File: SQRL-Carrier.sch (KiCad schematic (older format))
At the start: 59 parts, among them J1 M.2_M-key, J2 PCIE-164-02-F-D-RA, J3 4-Pin Molex, U1 DSC1104, U2 SI53322, U3 TPS563231, U4 TPS563231, U5 spoolqueue_logo

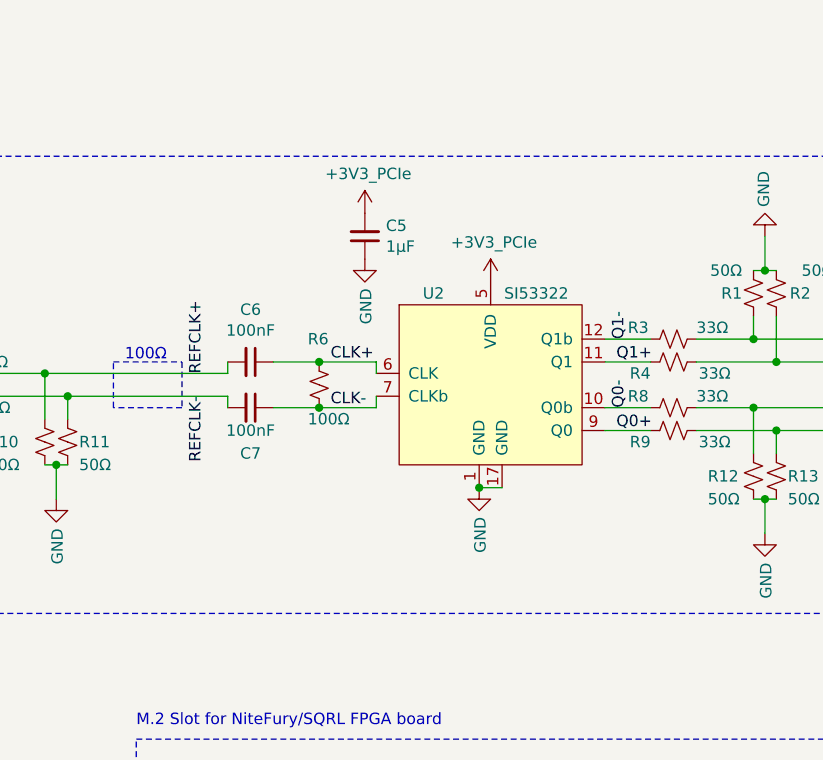
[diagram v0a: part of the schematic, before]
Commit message: Hardware revision 2
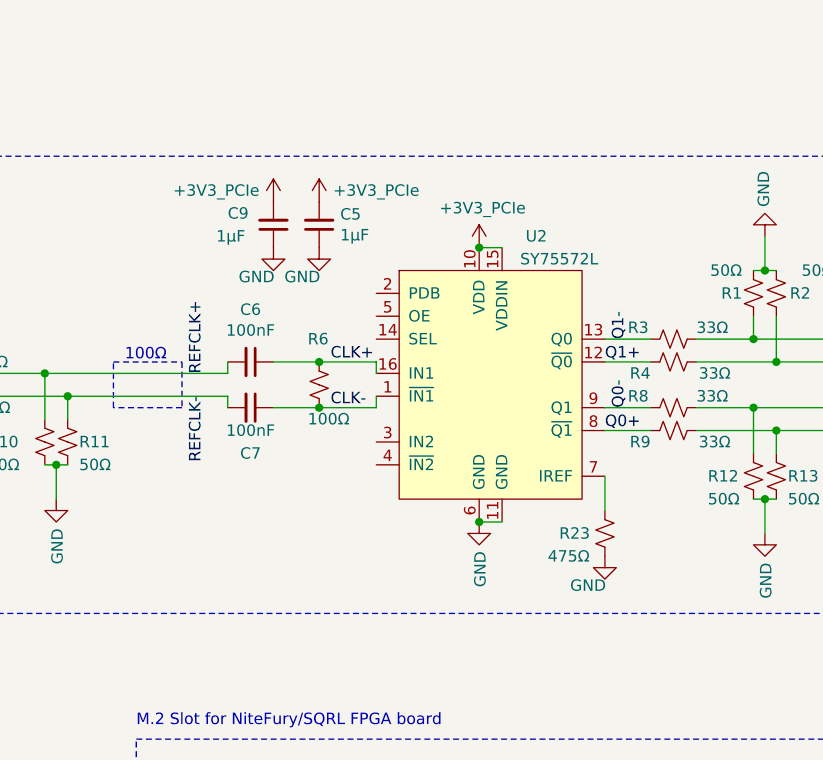
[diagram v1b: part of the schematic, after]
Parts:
- removed U2: SI53322, Package_DFN_QFN:VQFN-16-1EP_3x3mm_P0.5mm_EP1.68x1.68mm_ThermalVias, symbol PCIe_Clock:SI53322
- added C9: 1μF, Capacitor_SMD:C_0402_1005Metric, symbol Device:C_Small
- added R23: 475Ω, Resistor_SMD:R_0402_1005Metric, symbol Device:R_Small_US
- added U2: SY75572L, Package_DFN_QFN:VQFN-16-1EP_3x3mm_P0.5mm_EP1.45x1.45mm, symbol PCIe_Clock:SY75572L
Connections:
- net +3V3_PCIe: now also C9.2, U2.10 (VDD), U2.15 (VDDIN)
- net CLK+: now also U2.16 (IN1)
- net CLK-: now also U2.1 (~IN1~)
- net GND: now also C9.1, R23.2, U2.11 (GND), U2.6 (GND)
- net Q0+: now also U2.8 (~Q1~)
- net Q0-: now also U2.9 (Q1)
- net Q1+: now also U2.12 (~Q0~)
- net Q1-: now also U2.13 (Q0)
- new net: R23.1, U2.7 (IREF)
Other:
- moved on the sheet: C5
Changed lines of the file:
@@
 L power:GND #PWR0114
 U 1 1 5EADCD70
-P 8000 3450
-F 0 "#PWR0114" H 8000 3200 50  0001 C CNN
-F 1 "GND" V 8005 3322 50  0000 R CNN
-F 2 "" H 8000 3450 50  0001 C CNN
-F 3 "" H 8000 3450 50  0001 C CNN
-	1    8000 3450
+P 8000 3600
+F 0 "#PWR0114" H 8000 3350 50  0001 C CNN
+F 1 "GND" V 8005 3472 50  0000 R CNN
+F 2 "" H 8000 3600 50  0001 C CNN
+F 3 "" H 8000 3600 50  0001 C CNN
+	1    8000 3600
 	1    0    0    -1
 $EndComp
@@
 Wire Wire Line
 	11200 6000 11300 6000
-$Comp
-L PCIe_Clock:SI53322 U2
-U 1 1 5EB6B52B
-P 8050 3000
-F 0 "U2" H 7800 3400 50  0000 C CNN
-F 1 "SI53322" H 8250 3400 50  0000 C CNN
-F 2 "Package_DFN_QFN:VQFN-16-1EP_3x3mm_P0.5mm_EP1.68x1.68mm_ThermalVias" H 8050 3000 50  0001 C CNN
-F 3 "" H 8050 3000 50  0001 C CNN
-	1    8050 3000
-	1    0    0    -1
-$EndComp
-Wire Wire Line
-	8000 3450 8100 3450
-Connection ~ 8000 3450
+Wire Wire Line
+	8000 3600 8100 3600
 $Comp
 L power:GND #PWR0115
@@
 	6200 3050 6900 3050
 $Comp
-L Device:R_Small_US R12
-U 1 1 5EBAFF1E
-P 9200 3400
-F 0 "R12" H 9000 3400 50  0000 L CNN
-F 1 "50Ω" H 9000 3300 50  0000 L CNN
-F 2 "Resistor_SMD:R_0402_1005Metric" H 9200 3400 50  0001 C CNN
-F 3 "~" H 9200 3400 50  0001 C CNN
-	1    9200 3400
-	1    0    0    -1
-$EndComp
-$Comp
-L Device:R_Small_US R13
-U 1 1 5EBAFF24
-P 9300 3400
-F 0 "R13" H 9350 3400 50  0000 L CNN
-F 1 "50Ω" H 9350 3300 50  0000 L CNN
-F 2 "Resistor_SMD:R_0402_1005Metric" H 9300 3400 50  0001 C CNN
-F 3 "~" H 9300 3400 50  0001 C CNN
-	1    9300 3400
-	1    0    0    -1
-$EndComp
-$Comp
 L power:GND #PWR0117
 U 1 1 5EBAFF2A
@@
 	9200 3500 9250 3500
 Connection ~ 9250 3500
-$Comp
-L Device:R_Small_US R8
-U 1 1 5EBAFF34
-P 8850 3100
-F 0 "R8" V 8800 2900 50  0000 L CNN
-F 1 "33Ω" V 8800 3200 50  0000 L CNN
-F 2 "Resistor_SMD:R_0402_1005Metric" H 8850 3100 50  0001 C CNN
-F 3 "~" H 8850 3100 50  0001 C CNN
-	1    8850 3100
-	0    1    1    0
-$EndComp
-$Comp
-L Device:R_Small_US R9
-U 1 1 5EBAFF3A
-P 8850 3200
-F 0 "R9" V 8800 3300 50  0000 L CNN
-F 1 "33Ω" V 8800 2950 50  0000 L CNN
-F 2 "Resistor_SMD:R_0402_1005Metric" H 8850 3200 50  0001 C CNN
-F 3 "~" H 8850 3200 50  0001 C CNN
-	1    8850 3200
-	0    -1   -1   0
-$EndComp
 Wire Wire Line
 	8550 3100 8750 3100
@@
 Wire Wire Line
 	9300 3200 10050 3200
-$Comp
-L Device:R_Small_US R2
-U 1 1 5EBC0DFE
-P 9300 2600
-F 0 "R2" H 9150 2600 50  0000 L CNN
-F 1 "50Ω" H 9050 2500 50  0000 L CNN
-F 2 "Resistor_SMD:R_0402_1005Metric" H 9300 2600 50  0001 C CNN
-F 3 "~" H 9300 2600 50  0001 C CNN
-	1    9300 2600
-	-1   0    0    1
-$EndComp
-$Comp
-L Device:R_Small_US R1
-U 1 1 5EBC0E04
-P 9200 2600
-F 0 "R1" H 9250 2600 50  0000 L CNN
-F 1 "50Ω" H 9250 2500 50  0000 L CNN
-F 2 "Resistor_SMD:R_0402_1005Metric" H 9200 2600 50  0001 C CNN
-F 3 "~" H 9200 2600 50  0001 C CNN
-	1    9200 2600
-	-1   0    0    1
-$EndComp
 $Comp
 L power:GND #PWR0118
@@
 Wire Wire Line
 	9300 2900 10050 2900
-$Comp
-L Device:R_Small_US R4
-U 1 1 5EBC0E14
-P 8850 2900
-F 0 "R4" V 8800 3000 50  0000 L CNN
-F 1 "33Ω" V 8800 2650 50  0000 L CNN
-F 2 "Resistor_SMD:R_0402_1005Metric" H 8850 2900 50  0001 C CNN
-F 3 "~" H 8850 2900 50  0001 C CNN
-	1    8850 2900
-	0    -1   -1   0
-$EndComp
 Wire Wire Line
 	8750 2900 8550 2900
 Wire Wire Line
 	8550 2800 8750 2800
-$Comp
-L Device:R_Small_US R3
-U 1 1 5EBC0E1A
-P 8850 2800
-F 0 "R3" V 8800 2600 50  0000 L CNN
-F 1 "33Ω" V 8800 2900 50  0000 L CNN
-F 2 "Resistor_SMD:R_0402_1005Metric" H 8850 2800 50  0001 C CNN
-F 3 "~" H 8850 2800 50  0001 C CNN
-	1    8850 2800
-	0    1    1    0
-$EndComp
 Wire Notes Line
 	9550 3050 9850 3050
@@
 L Device:C_Small C5
 U 1 1 5EEDCC6E
-P 7500 2350
-F 0 "C5" H 7408 2304 50  0000 R CNN
-F 1 "1μF" H 7408 2395 50  0000 R CNN
-F 2 "Capacitor_SMD:C_0402_1005Metric" H 7500 2350 50  0001 C CNN
-F 3 "~" H 7500 2350 50  0001 C CNN
-	1    7500 2350
+P 7300 2300
+F 0 "C5" H 7208 2254 50  0000 R CNN
+F 1 "1μF" H 7208 2345 50  0000 R CNN
+F 2 "Capacitor_SMD:C_0402_1005Metric" H 7300 2300 50  0001 C CNN
+F 3 "~" H 7300 2300 50  0001 C CNN
+	1    7300 2300
 	-1   0    0    1
-$EndComp
-$Comp
-L power:GND #PWR0225
-U 1 1 5EEDCC74
-P 7500 2450
-F 0 "#PWR0225" H 7500 2200 50  0001 C CNN
-F 1 "GND" V 7505 2322 50  0000 R CNN
-F 2 "" H 7500 2450 50  0001 C CNN
-F 3 "" H 7500 2450 50  0001 C CNN
-	1    7500 2450
-	1    0    0    -1
 $EndComp
 $Comp
 L Carrier_power:+3V3_PCIe #PWR0226
 U 1 1 5EEE3C1E
-P 8050 2550
-F 0 "#PWR0226" H 8050 2400 50  0001 C CNN
-F 1 "+3V3_PCIe" H 8065 2723 50  0000 C CNN
-F 2 "" H 8050 2550 50  0001 C CNN
-F 3 "" H 8050 2550 50  0001 C CNN
-	1    8050 2550
+P 8000 2400
+F 0 "#PWR0226" H 8000 2250 50  0001 C CNN
+F 1 "+3V3_PCIe" H 8015 2573 50  0000 C CNN
+F 2 "" H 8000 2400 50  0001 C CNN
+F 3 "" H 8000 2400 50  0001 C CNN
+	1    8000 2400
 	1    0    0    -1
 $EndComp
@@
 L Carrier_power:+3V3_PCIe #PWR0227
 U 1 1 5EEE78B2
-P 7500 2250
-F 0 "#PWR0227" H 7500 2100 50  0001 C CNN
-F 1 "+3V3_PCIe" H 7515 2423 50  0000 C CNN
-F 2 "" H 7500 2250 50  0001 C CNN
-F 3 "" H 7500 2250 50  0001 C CNN
-	1    7500 2250
+P 7300 2200
+F 0 "#PWR0227" H 7300 2050 50  0001 C CNN
+F 1 "+3V3_PCIe" H 7550 2250 50  0000 C CNN
+F 2 "" H 7300 2200 50  0001 C CNN
+F 3 "" H 7300 2200 50  0001 C CNN
+	1    7300 2200
 	1    0    0    -1
 $EndComp
@@
 Text Label 8650 2800 1    50   ~ 0
 Q1-
-Text Label 8600 2900 0    50   ~ 0
+Text Label 8550 2900 0    50   ~ 0
 Q1+
-Text Label 8600 3200 0    50   ~ 0
+Text Label 8550 3200 0    50   ~ 0
 Q0+
 Text Label 8650 3100 1    50   ~ 0
@@
 	1    0    0    -1
 $EndComp
+$Comp
+L PCIe_Clock:SY75572L U2
+U 1 1 5F5400E1
+P 8050 3000
+F 0 "U2" H 8250 3650 50  0000 C CNN
+F 1 "SY75572L" H 8350 3550 50  0000 C CNN
+F 2 "Package_DFN_QFN:VQFN-16-1EP_3x3mm_P0.5mm_EP1.45x1.45mm" H 8050 3000 50  0001 C CNN
+F 3 "" H 8050 3000 50  0001 C CNN
+	1    8050 3000
+	1    0    0    -1
+$EndComp
+Connection ~ 8000 3600
+Wire Wire Line
+	8000 2400 8100 2400
+Connection ~ 8000 2400
+$Comp
+L Device:R_Small_US R23
+U 1 1 5F59552E
+P 8550 3650
+F 0 "R23" H 8350 3650 50  0000 L CNN
+F 1 "475Ω" H 8300 3550 50  0000 L CNN
+F 2 "Resistor_SMD:R_0402_1005Metric" H 8550 3650 50  0001 C CNN
+F 3 "~" H 8550 3650 50  0001 C CNN
+	1    8550 3650
+	1    0    0    -1
+$EndComp
+$Comp
+L power:GND #PWR0240
+U 1 1 5F597145
+P 8550 3750
+F 0 "#PWR0240" H 8550 3500 50  0001 C CNN
+F 1 "GND" H 8555 3622 50  0000 R CNN
+F 2 "" H 8550 3750 50  0001 C CNN
+F 3 "" H 8550 3750 50  0001 C CNN
+	1    8550 3750
+	1    0    0    -1
+$EndComp
+Wire Wire Line
+	8550 3550 8550 3400
+$Comp
+L Device:R_Small_US R8
+U 1 1 5EBAFF34
+P 8850 3100
+F 0 "R8" V 8800 2900 50  0000 L CNN
+F 1 "33Ω" V 8800 3200 50  0000 L CNN
+F 2 "Resistor_SMD:R_0402_1005Metric" H 8850 3100 50  0001 C CNN
+F 3 "~" H 8850 3100 50  0001 C CNN
+	1    8850 3100
+	0    1    1    0
+$EndComp
+$Comp
+L Device:R_Small_US R9
+U 1 1 5EBAFF3A
+P 8850 3200
+F 0 "R9" V 8800 3300 50  0000 L CNN
+F 1 "33Ω" V 8800 2950 50  0000 L CNN
+F 2 "Resistor_SMD:R_0402_1005Metric" H 8850 3200 50  0001 C CNN
+F 3 "~" H 8850 3200 50  0001 C CNN
+	1    8850 3200
+	0    -1   -1   0
+$EndComp
+$Comp
+L Device:R_Small_US R13
+U 1 1 5EBAFF24
+P 9300 3400
+F 0 "R13" H 9350 3400 50  0000 L CNN
+F 1 "50Ω" H 9350 3300 50  0000 L CNN
+F 2 "Resistor_SMD:R_0402_1005Metric" H 9300 3400 50  0001 C CNN
+F 3 "~" H 9300 3400 50  0001 C CNN
+	1    9300 3400
+	1    0    0    -1
+$EndComp
+$Comp
+L Device:R_Small_US R12
+U 1 1 5EBAFF1E
+P 9200 3400
+F 0 "R12" H 9000 3400 50  0000 L CNN
+F 1 "50Ω" H 9000 3300 50  0000 L CNN
+F 2 "Resistor_SMD:R_0402_1005Metric" H 9200 3400 50  0001 C CNN
+F 3 "~" H 9200 3400 50  0001 C CNN
+	1    9200 3400
+	1    0    0    -1
+$EndComp
+$Comp
+L Device:R_Small_US R2
+U 1 1 5EBC0DFE
+P 9300 2600
+F 0 "R2" H 9150 2600 50  0000 L CNN
+F 1 "50Ω" H 9050 2500 50  0000 L CNN
+F 2 "Resistor_SMD:R_0402_1005Metric" H 9300 2600 50  0001 C CNN
+F 3 "~" H 9300 2600 50  0001 C CNN
+	1    9300 2600
+	-1   0    0    1
+$EndComp
+$Comp
+L Device:R_Small_US R1
+U 1 1 5EBC0E04
+P 9200 2600
+F 0 "R1" H 9250 2600 50  0000 L CNN
+F 1 "50Ω" H 9250 2500 50  0000 L CNN
+F 2 "Resistor_SMD:R_0402_1005Metric" H 9200 2600 50  0001 C CNN
+F 3 "~" H 9200 2600 50  0001 C CNN
+	1    9200 2600
+	-1   0    0    1
+$EndComp
+$Comp
+L Device:R_Small_US R3
+U 1 1 5EBC0E1A
+P 8850 2800
+F 0 "R3" V 8800 2600 50  0000 L CNN
+F 1 "33Ω" V 8800 2900 50  0000 L CNN
+F 2 "Resistor_SMD:R_0402_1005Metric" H 8850 2800 50  0001 C CNN
+F 3 "~" H 8850 2800 50  0001 C CNN
+	1    8850 2800
+	0    1    1    0
+$EndComp
+$Comp
+L Device:R_Small_US R4
+U 1 1 5EBC0E14
+P 8850 2900
+F 0 "R4" V 8800 3000 50  0000 L CNN
+F 1 "33Ω" V 8800 2650 50  0000 L CNN
+F 2 "Resistor_SMD:R_0402_1005Metric" H 8850 2900 50  0001 C CNN
+F 3 "~" H 8850 2900 50  0001 C CNN
+	1    8850 2900
+	0    -1   -1   0
+$EndComp
+$Comp
+L power:GND #PWR0225
+U 1 1 5EEDCC74
+P 7300 2400
+F 0 "#PWR0225" H 7300 2150 50  0001 C CNN
+F 1 "GND" H 7305 2272 50  0000 R CNN
+F 2 "" H 7300 2400 50  0001 C CNN
+F 3 "" H 7300 2400 50  0001 C CNN
+	1    7300 2400
+	1    0    0    -1
+$EndComp
+$Comp
+L Device:C_Small C9
+U 1 1 5F66FF3D
+P 7100 2300
+F 0 "C9" H 7300 2250 50  0000 R CNN
+F 1 "1μF" H 7350 2350 50  0000 R CNN
+F 2 "Capacitor_SMD:C_0402_1005Metric" H 7100 2300 50  0001 C CNN
+F 3 "~" H 7100 2300 50  0001 C CNN
+	1    7100 2300
+	-1   0    0    1
+$EndComp
+$Comp
+L Carrier_power:+3V3_PCIe #PWR0242
+U 1 1 5F66FF43
+P 7100 2200
+F 0 "#PWR0242" H 7100 2050 50  0001 C CNN
+F 1 "+3V3_PCIe" H 6850 2250 50  0000 C CNN
+F 2 "" H 7100 2200 50  0001 C CNN
+F 3 "" H 7100 2200 50  0001 C CNN
+	1    7100 2200
+	1    0    0    -1
+$EndComp
+$Comp
+L power:GND #PWR0251
+U 1 1 5F66FF49
+P 7100 2400
+F 0 "#PWR0251" H 7100 2150 50  0001 C CNN
+F 1 "GND" H 7105 2272 50  0000 R CNN
+F 2 "" H 7100 2400 50  0001 C CNN
+F 3 "" H 7100 2400 50  0001 C CNN
+	1    7100 2400
+	1    0    0    -1
+$EndComp
